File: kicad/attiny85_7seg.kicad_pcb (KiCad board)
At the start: 2 copper layers, 55 x 65 mm, 23 parts, among them J1 Conn_01x06_Pin, J2 Conn_01x02_Pin, U1 ATtiny85, U2 CC56-12SURKWA, U3 74HC595, U4 74HC595

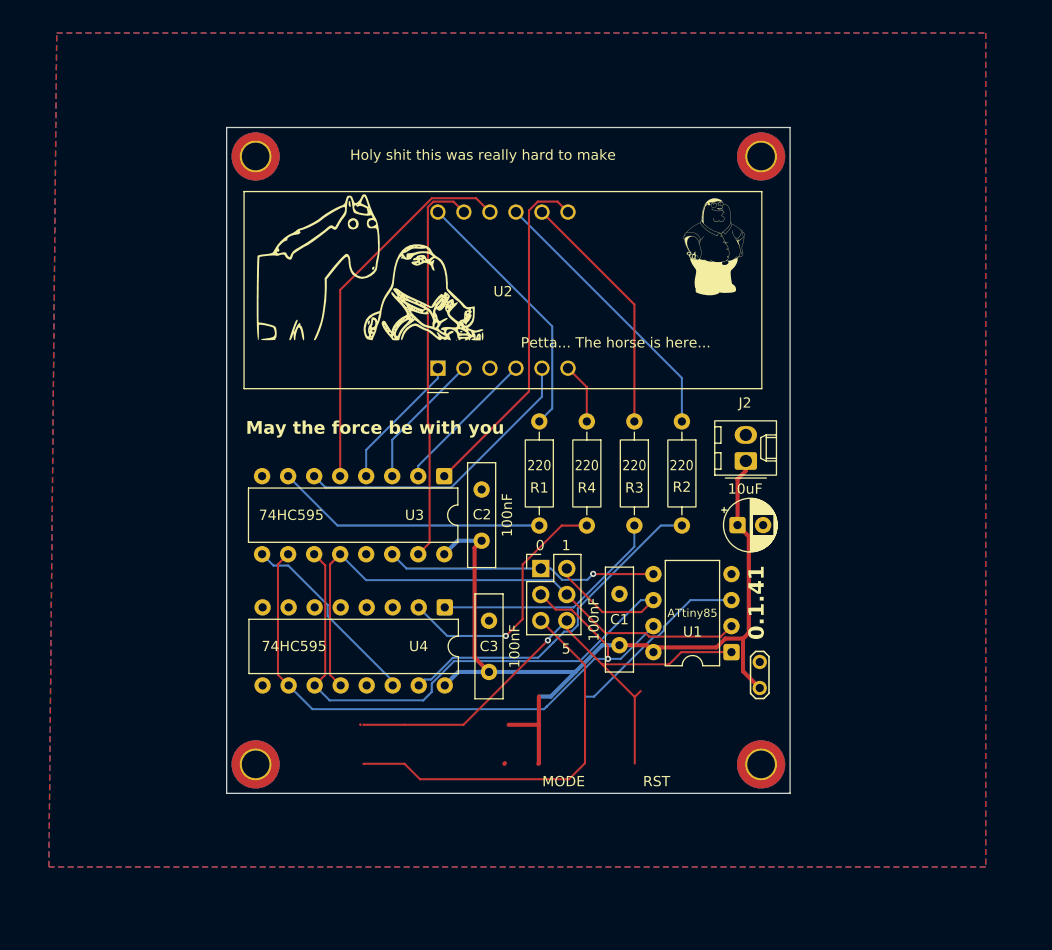
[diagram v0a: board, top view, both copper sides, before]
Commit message: v0.1.50
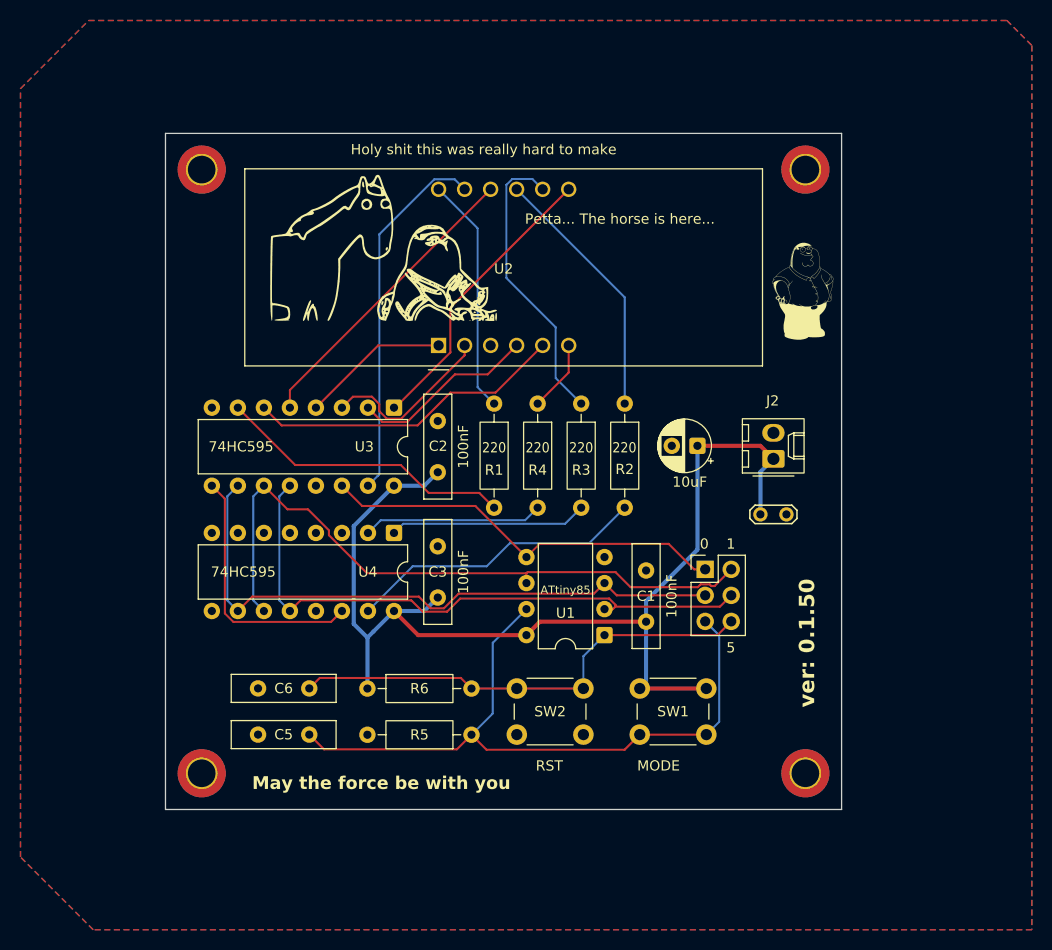
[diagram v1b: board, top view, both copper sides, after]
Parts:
- removed IMG2: KiCad-Logo_8mm_SilkScreen, Symbol:KiCad-Logo_8mm_SilkScreen
- added C5: 100nF, Capacitor_THT:C_Disc_D10.0mm_W2.5mm_P5.00mm, F.Cu at (126.4, 126.4)
- added C6: 100nF, Capacitor_THT:C_Disc_D10.0mm_W2.5mm_P5.00mm, F.Cu at (126.4, 121.9)
- added R5: 10k, Resistor_THT:R_Axial_DIN0207_L6.3mm_D2.5mm_P10.16mm_Horizontal, F.Cu at (142.3, 126.4)
- added R6: 10k, Resistor_THT:R_Axial_DIN0207_L6.3mm_D2.5mm_P10.16mm_Horizontal, F.Cu at (132.1, 121.9)
- added REF**: OSHW-Symbol_22.3x20mm_SilkScreen, Symbol:OSHW-Symbol_22.3x20mm_SilkScreen, B.Cu at (143.0, 103.0)
- added SW1: SW_Push, Button_Switch_THT:SW_PUSH_6mm, F.Cu at (165.2, 126.4)
- added SW2: SW_Push, Button_Switch_THT:SW_PUSH_6mm, F.Cu at (153.2, 126.4)
- moved H2 60.4 mm to (174.9, 130.1)
- moved H3 58.3 mm to (115.9, 71.2)
- moved H4 54.6 mm to (115.9, 130.1)
- moved H1 53.7 mm to (174.9, 71.2)
- moved IMG3 51.6 mm to (115.9, 82.3)
- moved TP1 16.9 mm to (170.5, 104.9), turned to 0 degrees
- moved J1 16.1 mm to (165.1, 110.2)
- moved U1 12.5 mm to (155.3, 116.7)
- moved IMG1 9.71 mm to (174.6, 83.1)
- moved C3 8.82 mm to (139.0, 113.0)
- moved U4 8.79 mm to (134.7, 106.7)
- moved C4 8.67 mm to (164.3, 98.2), turned to 180 degrees
- moved U3 8.29 mm to (134.7, 94.5)
- moved C2 7.94 mm to (139.0, 100.8)
- moved R2 5.85 mm to (157.2, 94.1)
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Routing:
- net /MODE: track 38.6 -> 67.8 mm
- net /SRCLR: track 81.9 -> 61.3 mm, vias 1 -> 0
- net VCC: track 87.3 -> 107.8 mm
- net /DATA: track 26.8 -> 39.9 mm, vias 1 -> 0
- net /RST: track 54.8 -> 46.6 mm, vias 1 -> 0
- net /QF: track 37.1 -> 29.4 mm
- net /D4: track 25.1 -> 17.6 mm, vias 1 -> 0
- net Net-(U3-QH'): track 18.9 -> 25.2 mm
- net /QB: track 34.0 -> 28.4 mm
- net Net-(U2-CC3): track 24.2 -> 28.6 mm
- net /RCLK: track 55.6 -> 59.6 mm
- net /D2: track 33.1 -> 29.2 mm
- net /QD: track 13.4 -> 17.2 mm
- net /D3: track 23.0 -> 19.3 mm
- net /QC: track 14.5 -> 18.2 mm
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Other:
- board size 55 x 65 mm -> 66 x 66 mm
- board text added: "ver: ${REVISION}"
- board text removed: "${REVISION}"
